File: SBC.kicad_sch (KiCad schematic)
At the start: 0 parts

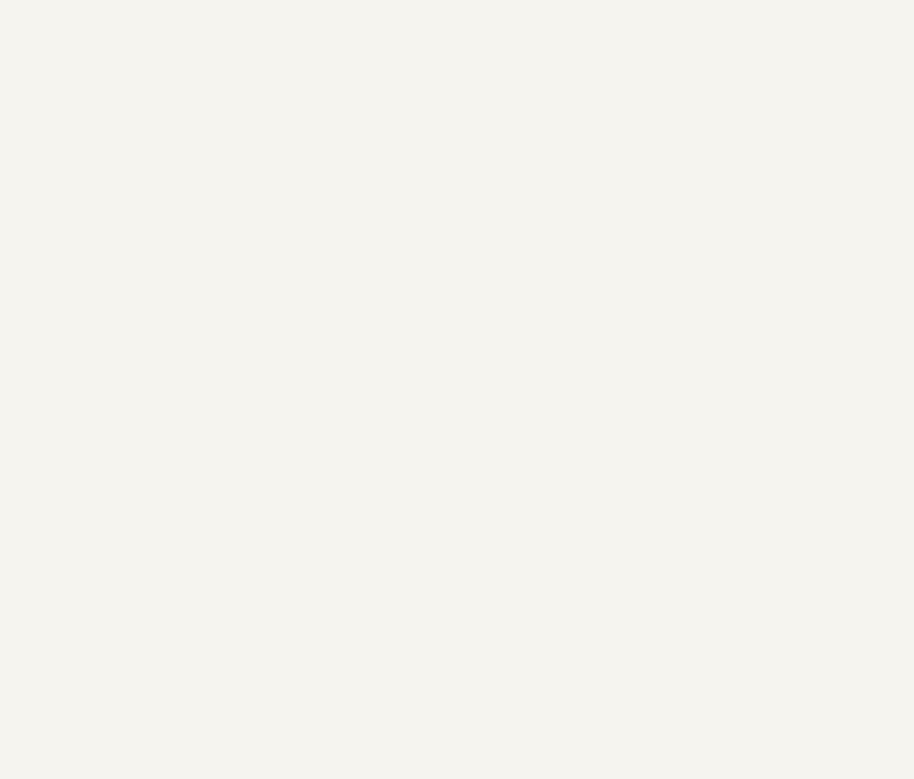
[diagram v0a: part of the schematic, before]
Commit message: More routing
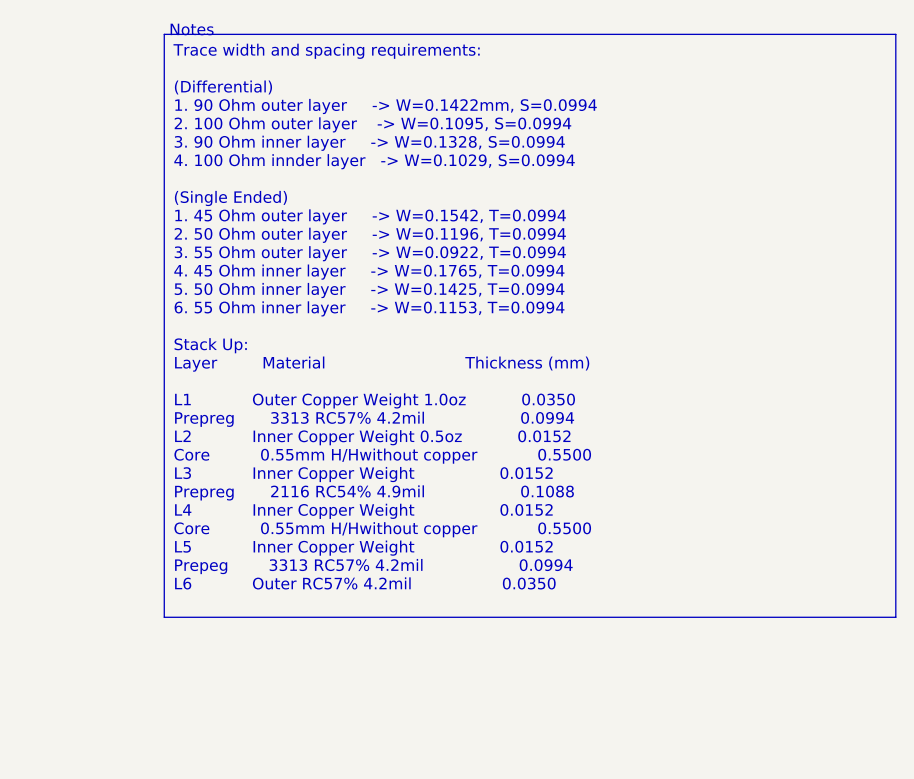
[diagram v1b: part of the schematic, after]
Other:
- note added: "Notes"
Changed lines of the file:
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@@
+		)
+	)
+	(text_box "Trace width and spacing requirements:\n\n(Differential)\n1. 90 Ohm outer layer     -> W=0.1422mm, S=0.0994\n2. 100 Ohm outer layer    -> W=0.1095, S=0.0994\n3. 90 Ohm inner layer     -> W=0.1328, S=0.0994\n4. 100 Ohm innder layer   -> W=0.1029, S=0.0994\n\n(Single Ended)\n1. 45 Ohm outer layer     -> W=0.1542, T=0.0994\n2. 50 Ohm outer layer     -> W=0.1196, T=0.0994\n3. 55 Ohm outer layer     -> W=0.0922, T=0.0994\n4. 45 Ohm inner layer     -> W=0.1765, T=0.0994\n5. 50 Ohm inner layer     -> W=0.1425, T=0.0994\n6. 55 Ohm inner layer     -> W=0.1153, T=0.0994\n\nStack Up:\nLayer         Material                            Thickness (mm)\n\nL1            Outer Copper Weight 1.0oz           0.0350\nPrepreg       3313 RC57% 4.2mil                   0.0994\nL2            Inner Copper Weight 0.5oz           0.0152\nCore          0.55mm H/Hwithout copper            0.5500\nL3            Inner Copper Weight                 0.0152\nPrepreg       2116 RC54% 4.9mil                   0.1088\nL4            Inner Copper Weight                 0.0152\nCore          0.55mm H/Hwithout copper            0.5500\nL5            Inner Copper Weight                 0.0152\nPrepeg        3313 RC57% 4.2mil                   0.0994\nL6            Outer RC57% 4.2mil                  0.0350"
+		(exclude_from_sim no)
+		(at 334.01 19.05 0)
+		(size 81.28 64.77)
+		(stroke
+			(width 0)
+			(type default)
+			(color 255 255 0 1)
+		)
+		(fill
+			(type none)
+		)
+		(effects
+			(font
+				(face "Courier New")
+				(size 1.27 1.27)
+				(color 255 255 0 1)
+			)
+			(justify left top)
+		)
+	)
+	(text "Notes"
+		(exclude_from_sim no)
+		(at 337.058 18.796 0)
+		(effects
+			(font
+				(face "Courier New")
+				(size 1.27 1.27)
+				(color 255 255 0 1)
+			)
 		)
 	)
